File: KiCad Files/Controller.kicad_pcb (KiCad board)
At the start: 2 copper layers, 28 parts, among them U1 ProS3D, U2 LT, U3 RT

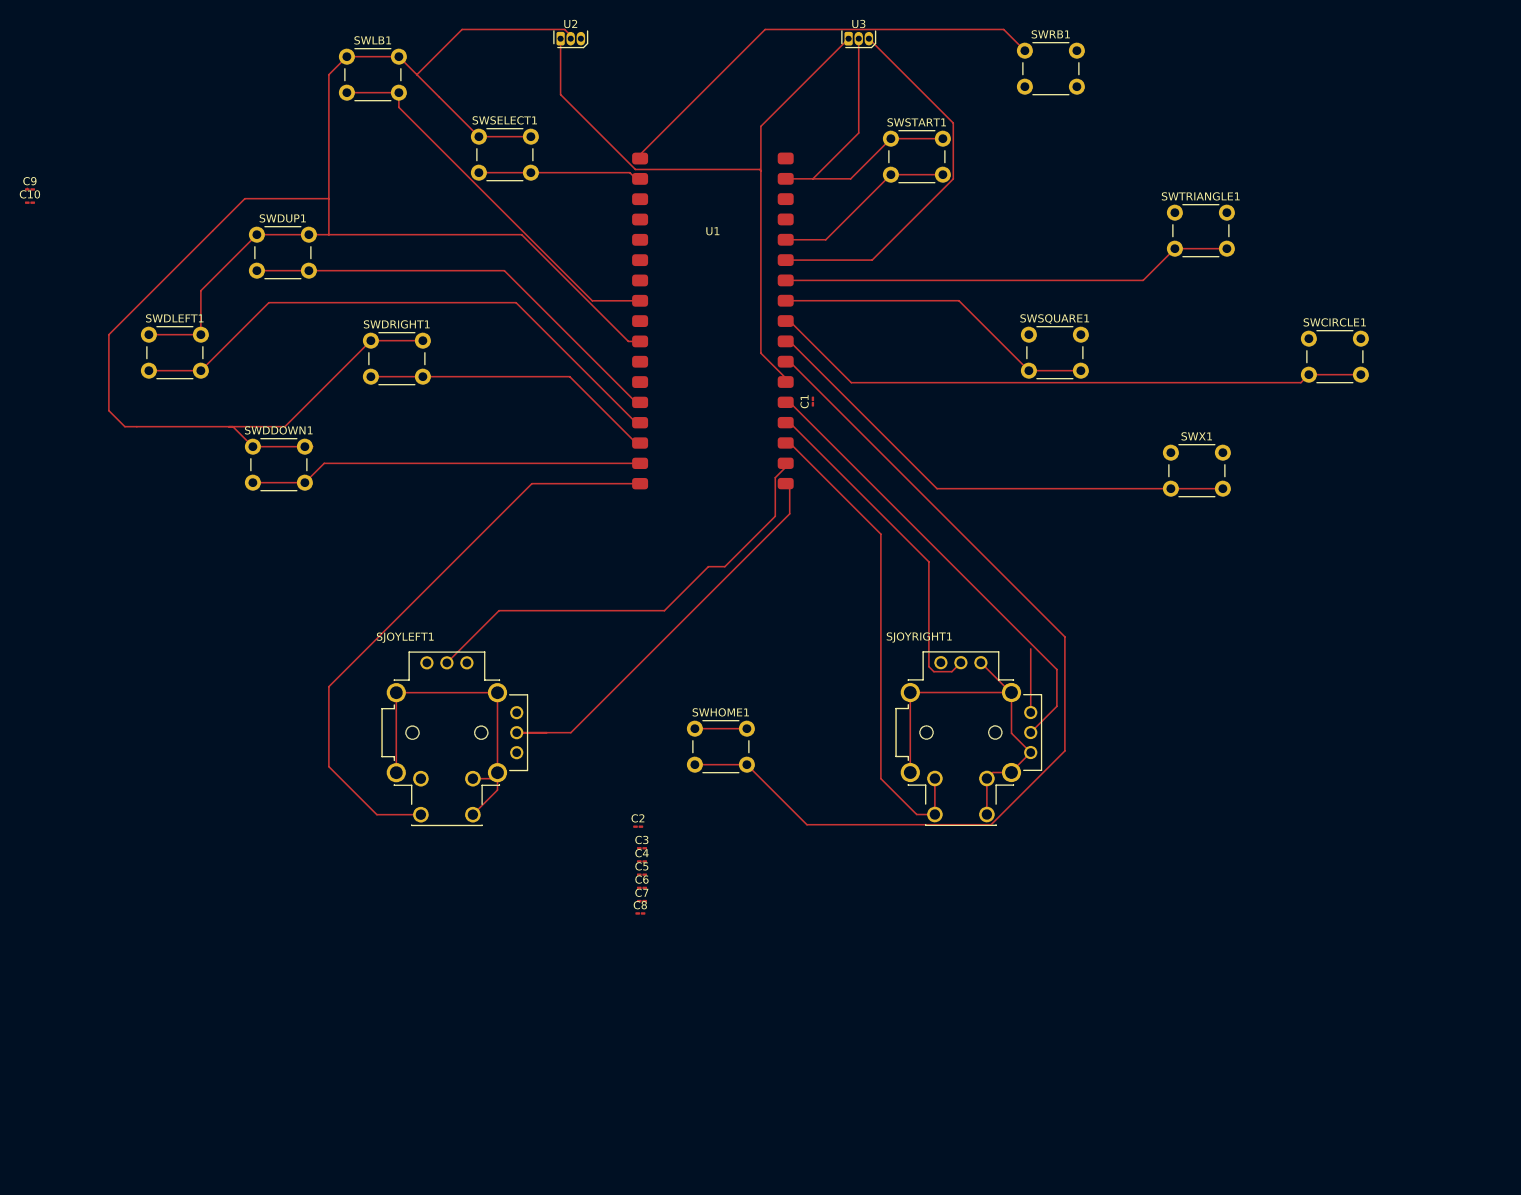
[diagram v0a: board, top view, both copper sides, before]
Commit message: Updated to current KiCad Design
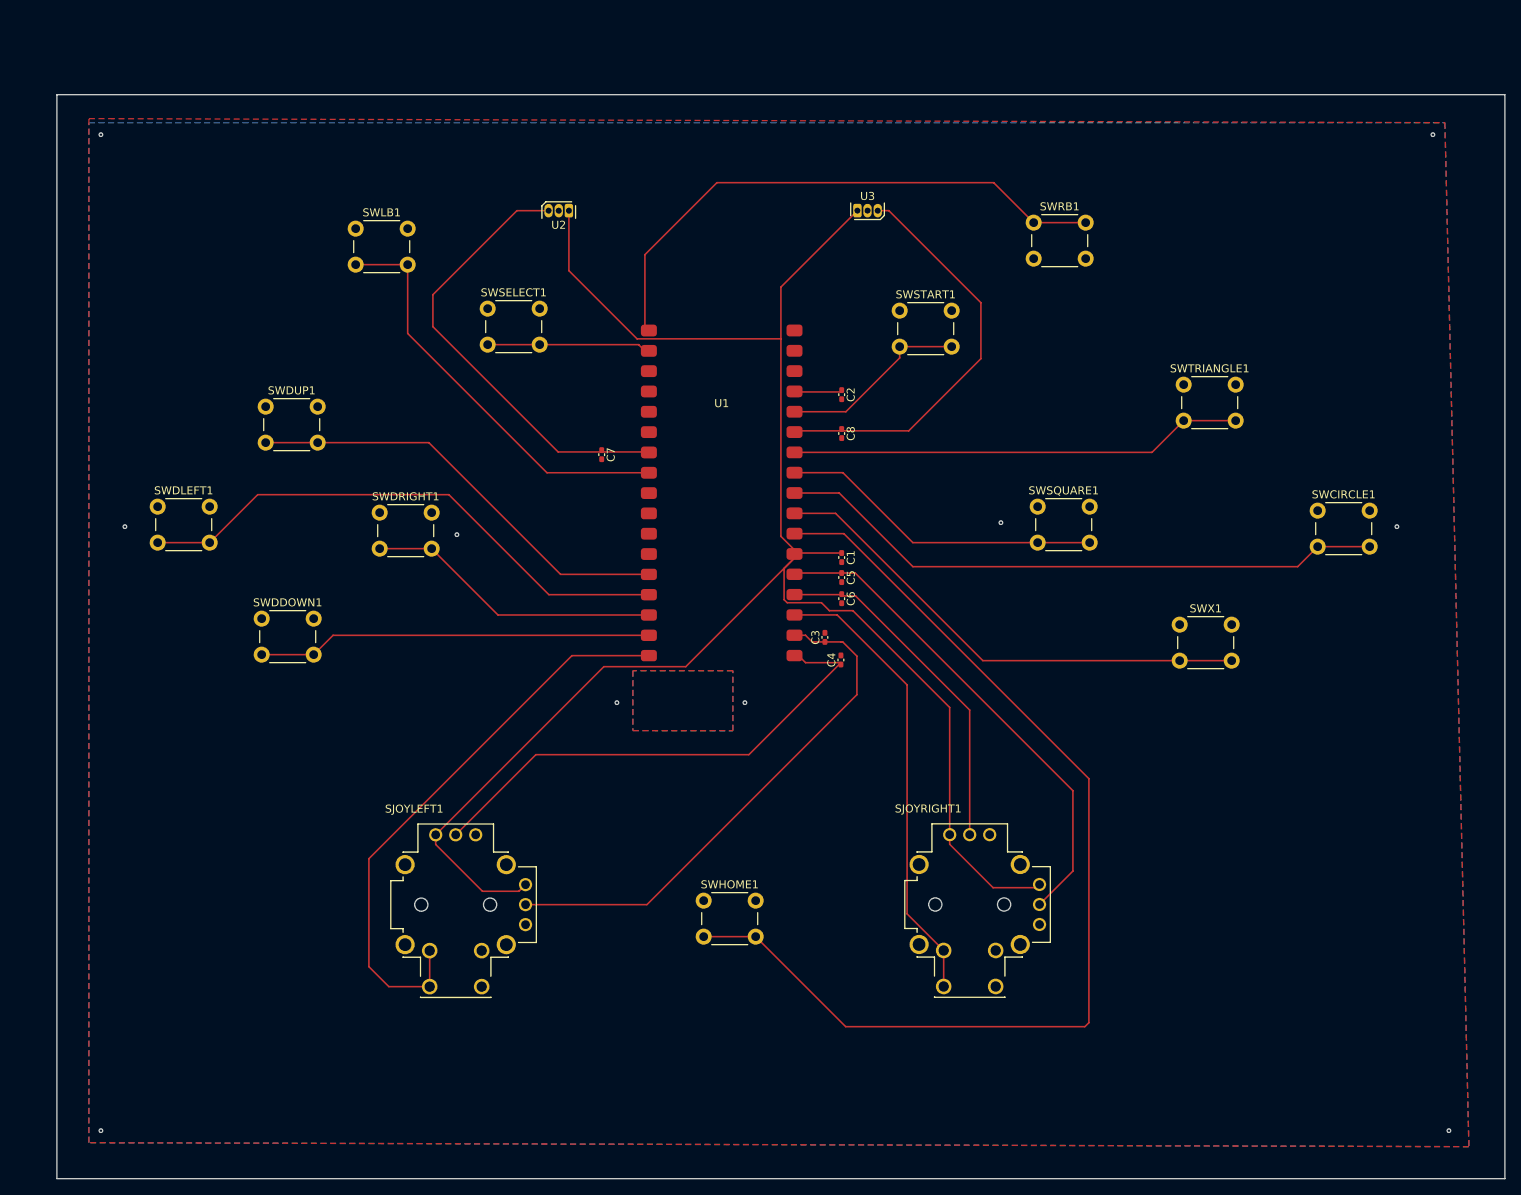
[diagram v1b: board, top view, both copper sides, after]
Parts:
- removed the C1 at (162.5, 68.9)
- removed the C2 at (140.7, 122.0)
- C1: renamed from C4; footprint Capacitor_SMD:C_01005_0402Metric_Pad0.57x0.30mm_HandSolder -> Capacitor_SMD:C_0402_1005Metric_Pad0.74x0.62mm_HandSolder
- C2: renamed from C3; footprint Capacitor_SMD:C_01005_0402Metric_Pad0.57x0.30mm_HandSolder -> Capacitor_SMD:C_0402_1005Metric_Pad0.74x0.62mm_HandSolder
- C3: renamed from C5; footprint Capacitor_SMD:C_01005_0402Metric_Pad0.57x0.30mm_HandSolder -> Capacitor_SMD:C_0402_1005Metric_Pad0.74x0.62mm_HandSolder
- C4: renamed from C6; footprint Capacitor_SMD:C_01005_0402Metric_Pad0.57x0.30mm_HandSolder -> Capacitor_SMD:C_0402_1005Metric_Pad0.74x0.62mm_HandSolder
- C5: renamed from C7; footprint Capacitor_SMD:C_01005_0402Metric_Pad0.57x0.30mm_HandSolder -> Capacitor_SMD:C_0402_1005Metric_Pad0.74x0.62mm_HandSolder
- C6: renamed from C8; footprint Capacitor_SMD:C_01005_0402Metric_Pad0.57x0.30mm_HandSolder -> Capacitor_SMD:C_0402_1005Metric_Pad0.74x0.62mm_HandSolder
- C7: renamed from C9; footprint Capacitor_SMD:C_01005_0402Metric_Pad0.57x0.30mm_HandSolder -> Capacitor_SMD:C_0402_1005Metric_Pad0.74x0.62mm_HandSolder
- C8: renamed from C10; footprint Capacitor_SMD:C_01005_0402Metric_Pad0.57x0.30mm_HandSolder -> Capacitor_SMD:C_0402_1005Metric_Pad0.74x0.62mm_HandSolder
- moved C8 105.5 mm to (166.1, 72.9), turned to -90 degrees
- moved C7 78.8 mm to (136.1, 75.5), turned to -90 degrees
- moved C2 62.0 mm to (166.1, 68.0), turned to -90 degrees
- moved C5 47.5 mm to (166.1, 90.9), turned to -90 degrees
- moved C6 46.7 mm to (166.1, 93.5), turned to -90 degrees
- moved C1 45.5 mm to (166.1, 88.4), turned to -90 degrees
- moved C4 37.8 mm to (166.0, 101.2), turned to 90 degrees
- moved C3 37.5 mm to (164.0, 98.3), turned to 90 degrees
- moved U2 21.5 mm to (132.0, 45.0), turned to 180 degrees
- moved SJOYRIGHT1 21.5 mm to (182.1, 131.7)
- moved SWLB1 21.5 mm to (105.3, 47.2)
- moved SWRB1 21.5 mm to (190.1, 46.5)
- moved SWSELECT1 21.5 mm to (121.8, 57.2)
- moved SWSTART1 21.5 mm to (173.3, 57.5)
- moved U3 21.5 mm to (168.1, 45.0)
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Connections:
- U1 pad 16: /JoyLeftY -> /JoyLeftX
- U1 pad 17: /JoyLeftX -> /JoyLeftY
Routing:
- net GND: track 386.5 -> 0.00 mm, vias 0 -> 10
- net /3V3Switched: track 92.9 -> 229.5 mm
- net /LT: track 0.55 -> 55.8 mm
- net /Home: track 116.1 -> 132.5 mm
- net /RB: track 56.4 -> 70.4 mm
- net /JoyLeftX: track 53.0 -> 65.5 mm
- net /JoyLeftY: track 56.0 -> 62.7 mm
- net /JoyRightX: track 56.5 -> 61.9 mm
- net /3V3: track 0.00 -> 5.43 mm
- net /RT: track 46.6 -> 51.3 mm
- net /LB: track 48.0 -> 52.0 mm
- net /R3: track 59.8 -> 56.8 mm
- net /DLEFT: track 70.6 -> 68.6 mm
- net /L3: track 72.9 -> 71.6 mm
- net /Circle: track 75.0 -> 76.3 mm
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- added copper zone on B.Cu, net GND
- added copper zone on F.Cu, net GND
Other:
- board outline added: 181 x 135.5 mm
